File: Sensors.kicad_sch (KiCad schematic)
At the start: 7 parts, among them J1 Conn_01x03_Socket, J4 Conn_01x03_Socket, J5 Conn_01x02_Socket

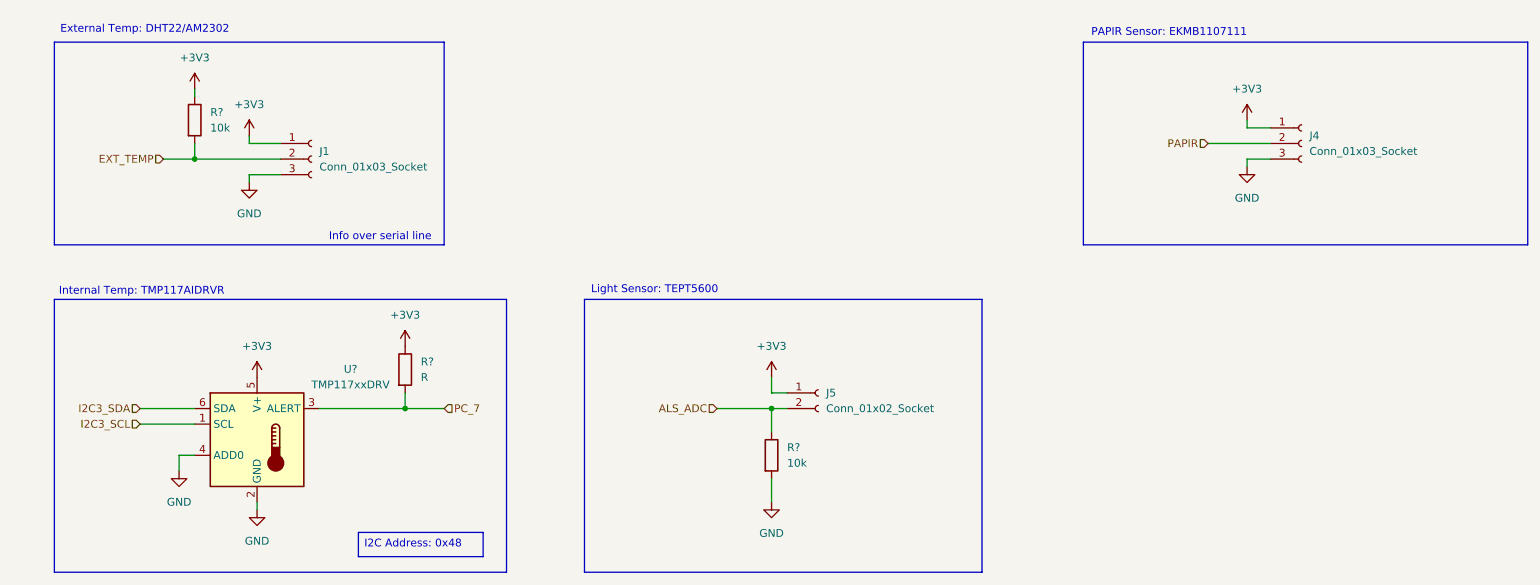
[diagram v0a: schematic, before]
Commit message: wait
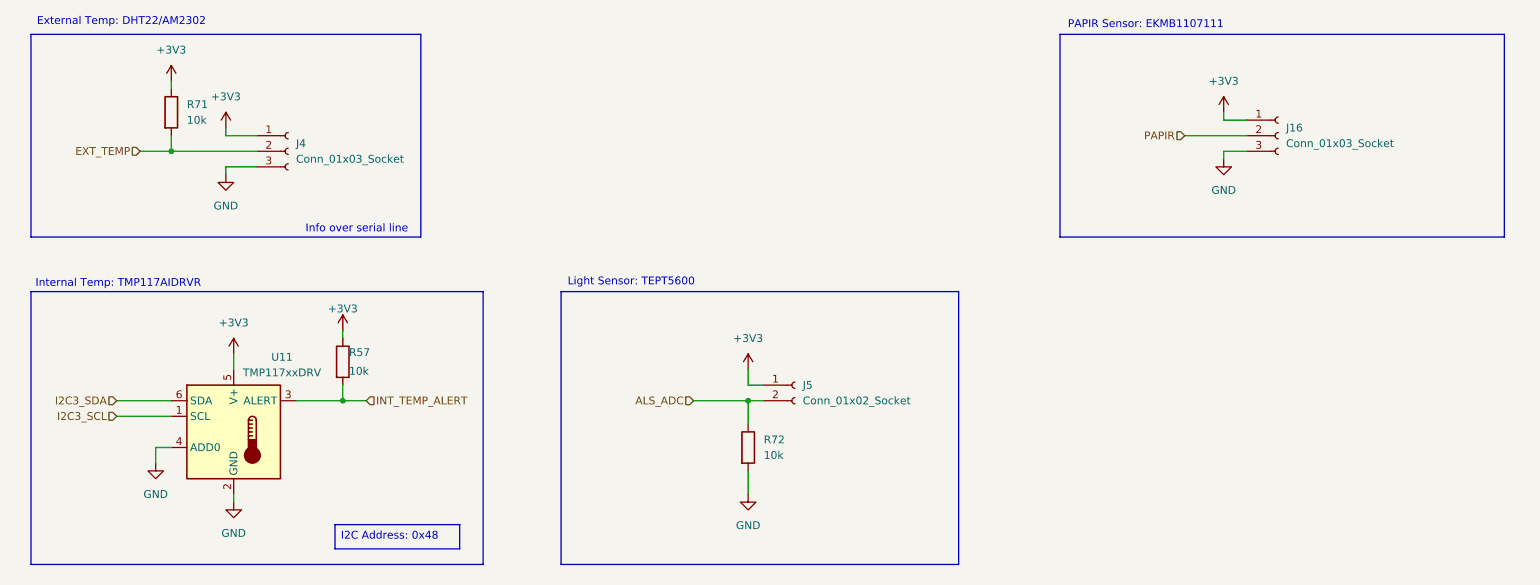
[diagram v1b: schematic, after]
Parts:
- removed J1: Conn_01x03_Socket, Package_SO:HTSSOP-20-1EP_4.4x6.5mm_P0.65mm_EP3.4x6.5mm_ThermalVias, symbol Connector:Conn_01x03_Socket
- removed R? (x2): 10k, Resistor_SMD:R_0603_1608Metric, symbol Device:R
- removed R?: R, Package_SON:WSON-6-1EP_2x2mm_P0.65mm_EP1x1.6mm, symbol Device:R
- removed U?: TMP117xxDRV, Package_SON:WSON-6-1EP_2x2mm_P0.65mm_EP1x1.6mm, symbol Sensor_Temperature:TMP117xxDRV
- added J16: Conn_01x03_Socket, symbol Connector:Conn_01x03_Socket
- added R57, R71, R72: 10k, Resistor_SMD:R_0603_1608Metric, symbol Device:R
- added U11: TMP117xxDRV, Package_SON:WSON-6-1EP_2x2mm_P0.65mm_EP1x1.6mm, symbol Sensor_Temperature:TMP117xxDRV
- J4: footprint (none) -> Connector_PinHeader_2.54mm:PinHeader_1x03_P2.54mm_Vertical
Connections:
- net +3V3: now also J16.1 (Pin_1), R57.1, R71.1, U11.5 (V+)
- net ALS_ADC: now also R72.1
- net EXT_TEMP: now also J4.2 (Pin_2), R71.2
- net GND: now also J16.3 (Pin_3), R72.2, U11.2 (GND), U11.4 (ADD0)
- net I2C3_SCL: now also U11.1 (SCL)
- net I2C3_SDA: now also U11.6 (SDA)
- net PAPIR: now also J16.2 (Pin_2); no longer J4.2 (Pin_2)
- new net INT_TEMP_ALERT: R57.2, U11.3 (ALERT)
